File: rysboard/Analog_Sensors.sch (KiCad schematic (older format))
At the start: 25 parts, among them J14 BAT2_TH, J21 BAT3_TH, J22 BAT2_TH, J23 BAT2_TH, J8 BAT1_TH, Q10 DMP2075UFDB

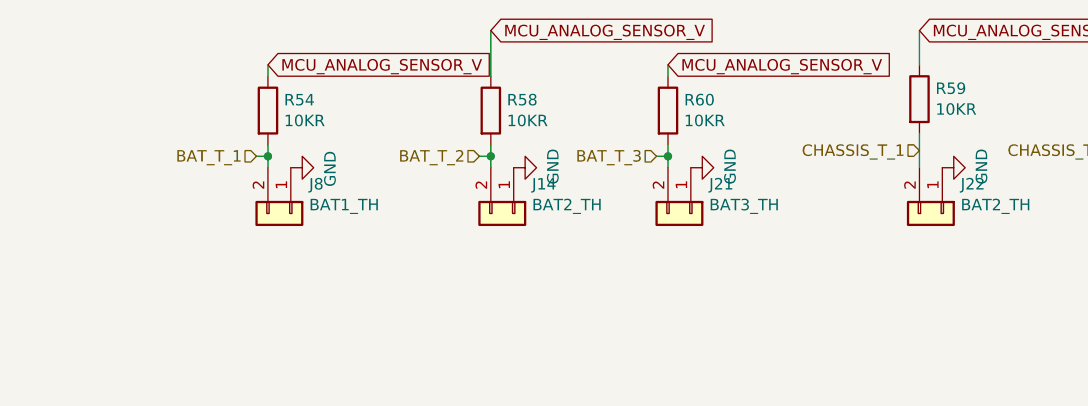
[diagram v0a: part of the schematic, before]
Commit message: cleanup and energy managment scheeme started
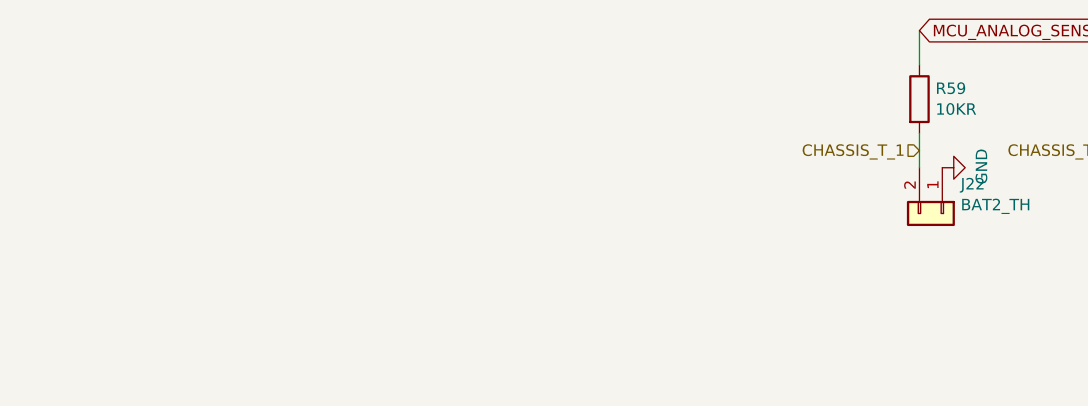
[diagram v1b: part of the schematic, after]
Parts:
- removed J14: BAT2_TH, symbol Connector_Generic:Conn_01x02
- removed J21: BAT3_TH, symbol Connector_Generic:Conn_01x02
- removed J8: BAT1_TH, symbol Connector_Generic:Conn_01x02
- removed R54, R58, R60: 10KR, Resistor_SMD:R_0603_1608Metric, symbol Device:R
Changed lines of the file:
@@
 Comment4 ""
 $EndDescr
-Text HLabel 3325 1300 0    50   Input ~ 0
-BAT_T_2
-Text HLabel 4100 1300 0    50   Input ~ 0
-BAT_T_3
 Text HLabel 3150 2875 0    50   Input ~ 0
 BOARD_T_1
@@
 Text HLabel 7850 4550 0    50   Input ~ 0
 V_BAT_C3
-$Comp
-L Connector_Generic:Conn_01x02 J8
-U 1 1 603EB5C9
-P 2500 1550
-F 0 "J8" V 2372 1630 50  0000 L CNN
-F 1 "BAT1_TH" V 2463 1630 50  0000 L CNN
-F 2 "" H 2500 1550 50  0001 C CNN
-F 3 "~" H 2500 1550 50  0001 C CNN
-	1    2500 1550
-	0    1    1    0
-$EndComp
-$Comp
-L Connector_Generic:Conn_01x02 J14
-U 1 1 603EBF1A
-P 3475 1550
-F 0 "J14" V 3347 1630 50  0000 L CNN
-F 1 "BAT2_TH" V 3438 1630 50  0000 L CNN
-F 2 "" H 3475 1550 50  0001 C CNN
-F 3 "~" H 3475 1550 50  0001 C CNN
-	1    3475 1550
-	0    1    1    0
-$EndComp
-$Comp
-L Connector_Generic:Conn_01x02 J21
-U 1 1 603EC2EC
-P 4250 1550
-F 0 "J21" V 4122 1630 50  0000 L CNN
-F 1 "BAT3_TH" V 4213 1630 50  0000 L CNN
-F 2 "" H 4250 1550 50  0001 C CNN
-F 3 "~" H 4250 1550 50  0001 C CNN
-	1    4250 1550
-	0    1    1    0
-$EndComp
-$Comp
-L power:GND #PWR050
-U 1 1 603ED9D9
-P 2500 1350
-F 0 "#PWR050" H 2500 1100 50  0001 C CNN
-F 1 "GND" H 2505 1177 50  0000 C CNN
-F 2 "" H 2500 1350 50  0001 C CNN
-F 3 "" H 2500 1350 50  0001 C CNN
-	1    2500 1350
-	0    -1   1    0
-$EndComp
-$Comp
-L power:GND #PWR053
-U 1 1 603EDE43
-P 3475 1350
-F 0 "#PWR053" H 3475 1100 50  0001 C CNN
-F 1 "GND" H 3480 1177 50  0000 C CNN
-F 2 "" H 3475 1350 50  0001 C CNN
-F 3 "" H 3475 1350 50  0001 C CNN
-	1    3475 1350
-	0    -1   -1   0
-$EndComp
-$Comp
-L power:GND #PWR054
-U 1 1 603EE031
-P 4250 1350
-F 0 "#PWR054" H 4250 1100 50  0001 C CNN
-F 1 "GND" H 4255 1177 50  0000 C CNN
-F 2 "" H 4250 1350 50  0001 C CNN
-F 3 "" H 4250 1350 50  0001 C CNN
-	1    4250 1350
-	0    -1   -1   0
-$EndComp
 Wire Wire Line
 	3150 2525 3150 2575
@@
 Text Notes 7750 3650 0    50   ~ 0
 0-15.086V\n
-Text HLabel 2350 1300 0    50   Input ~ 0
-BAT_T_1
-Wire Wire Line
-	2350 1300 2400 1300
-Wire Wire Line
-	2400 1300 2400 1350
-Wire Wire Line
-	2400 1300 2400 1250
-Connection ~ 2400 1300
-Wire Wire Line
-	3325 1300 3375 1300
-Wire Wire Line
-	3375 1300 3375 1250
-Wire Wire Line
-	3375 1300 3375 1350
-Connection ~ 3375 1300
-Wire Wire Line
-	4100 1300 4150 1300
-Wire Wire Line
-	4150 1300 4150 1250
-Wire Wire Line
-	4150 1300 4150 1350
-Connection ~ 4150 1300
 $Comp
 L Device:R R70
@@
 Text GLabel 8625 1800 1    50   Output ~ 0
 MCU_3.3V
-Wire Wire Line
-	2400 900  2400 950
-Wire Wire Line
-	4150 900  4150 950
 $Comp
 L Device:R R55
@@
 When not used, thermistors do not need to be powered on.
 $Comp
-L Device:R R54
-U 1 1 603FD549
-P 2400 1100
-F 0 "R54" H 2470 1146 50  0000 L CNN
-F 1 "10KR" H 2470 1055 50  0000 L CNN
-F 2 "Resistor_SMD:R_0603_1608Metric" V 2330 1100 50  0001 C CNN
-F 3 "~" H 2400 1100 50  0001 C CNN
-	1    2400 1100
-	1    0    0    -1
-$EndComp
-$Comp
-L Device:R R58
-U 1 1 603FD808
-P 3375 1100
-F 0 "R58" H 3445 1146 50  0000 L CNN
-F 1 "10KR" H 3445 1055 50  0000 L CNN
-F 2 "Resistor_SMD:R_0603_1608Metric" V 3305 1100 50  0001 C CNN
-F 3 "~" H 3375 1100 50  0001 C CNN
-	1    3375 1100
-	1    0    0    -1
-$EndComp
-$Comp
-L Device:R R60
-U 1 1 603FDA2E
-P 4150 1100
-F 0 "R60" H 4220 1146 50  0000 L CNN
-F 1 "10KR" H 4220 1055 50  0000 L CNN
-F 2 "Resistor_SMD:R_0603_1608Metric" V 4080 1100 50  0001 C CNN
-F 3 "~" H 4150 1100 50  0001 C CNN
-	1    4150 1100
-	1    0    0    -1
-$EndComp
-$Comp
 L rysboard:DMP2075UFDB Q10
 U 1 1 605EDFDE
@@
 Wire Wire Line
 	6150 1225 6150 1375
-Text HLabel 5250 1275 0    50   Input ~ 0
-CHASSIS_T_1
 Wire Wire Line
 	5250 1200 5250 1350
@@
 Text GLabel 5250 750  2    50   Input ~ 0
 MCU_ANALOG_SENSOR_V
-Text GLabel 4150 900  2    50   Input ~ 0
-MCU_ANALOG_SENSOR_V
-Text GLabel 3375 750  2    50   Input ~ 0
-MCU_ANALOG_SENSOR_V
-Wire Wire Line
-	3375 750  3375 950
-Text GLabel 2400 900  2    50   Input ~ 0
-MCU_ANALOG_SENSOR_V
 Wire Wire Line
 	5250 750  5250 900
 Text GLabel 3150 2525 0    50   Input ~ 0
 MCU_ANALOG_SENSOR_V
+Text HLabel 5250 1275 0    50   Input ~ 0
+CHASSIS_T_1
 $EndSCHEMATC
